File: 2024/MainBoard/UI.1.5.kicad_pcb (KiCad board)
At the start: 2 copper layers, 105.9 x 122.4 mm, 31 parts, among them J1 debug, Y2 Crystal_GND24

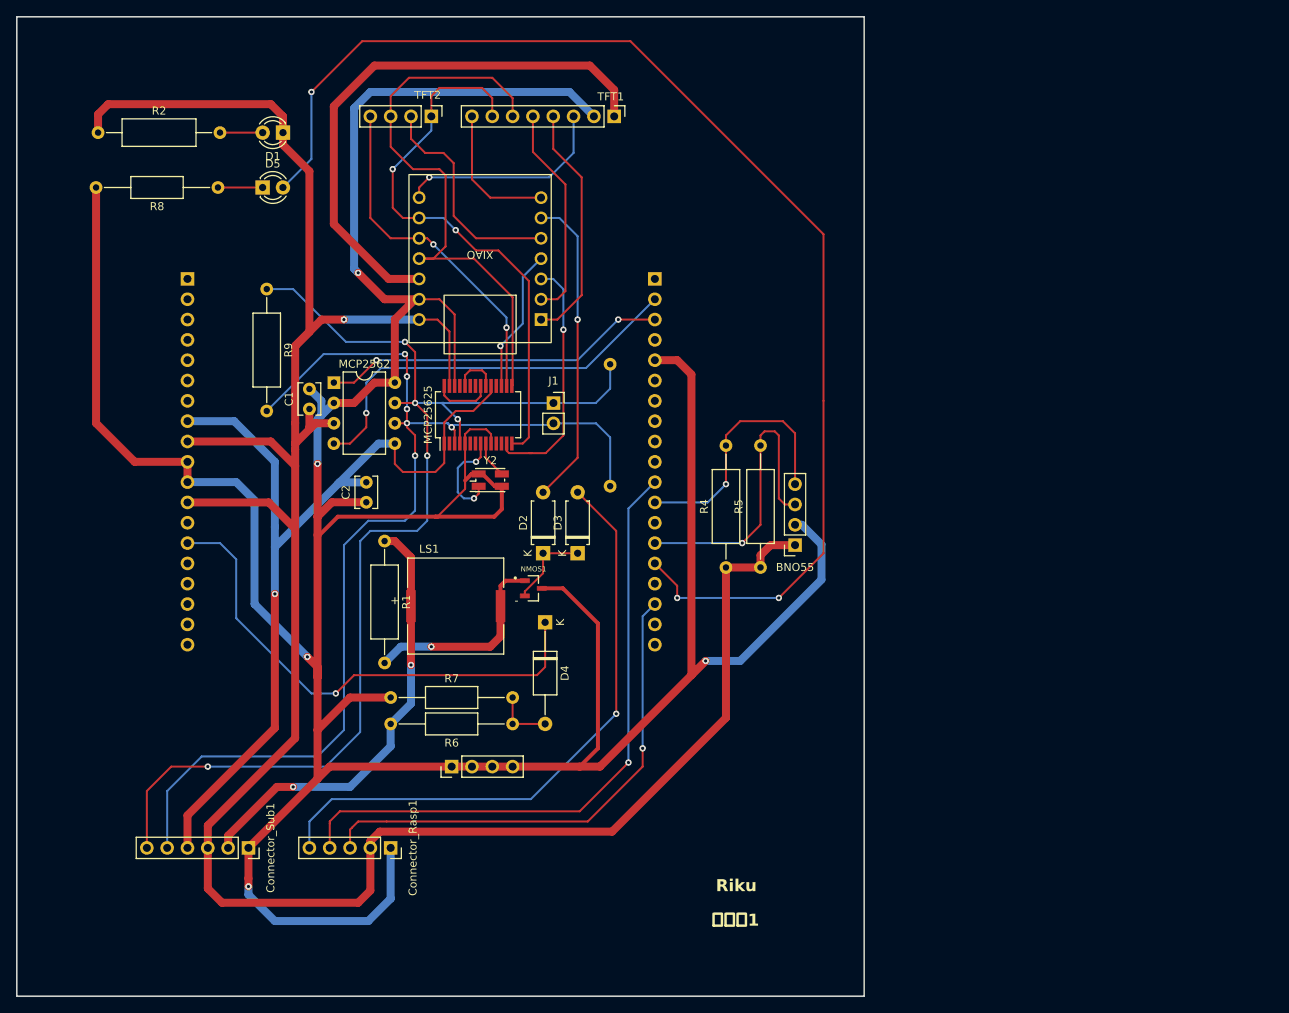
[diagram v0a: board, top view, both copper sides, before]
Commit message: アートワークした
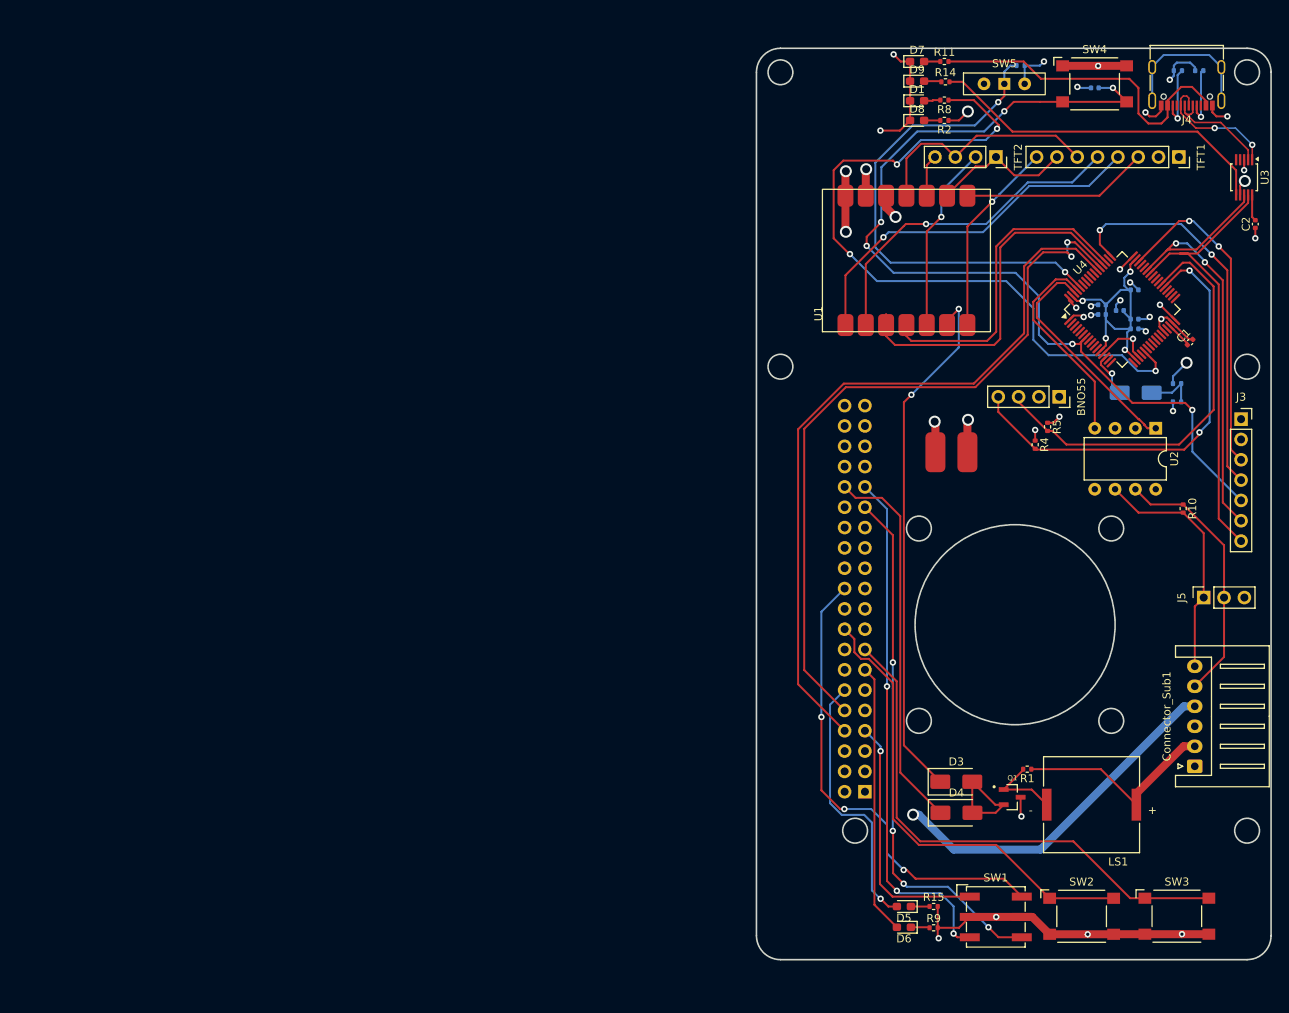
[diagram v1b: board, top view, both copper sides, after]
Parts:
- removed Connector_Rasp1: ~, Connector_PinSocket_2.54mm:PinSocket_1x05_P2.54mm_Vertical
- removed F446RE_CN10, F446RE_CN7: ~, Connector_PinSocket_2.54mm:PinSocket_1x19_P2.54mm_Vertical
- removed MCP2562: MCP2562-E-P, Package_DIP:DIP-8_W7.62mm
- removed MCP25625: MCP25625-x-SS, Package_SO:SSOP-28_5.3x10.2mm_P0.65mm
- removed NMOS1: BSS138, NMOS:SOT95P240X111-3N
- removed TFT3: ~, Connector_PinHeader_2.54mm:PinHeader_1x04_P2.54mm_Vertical
- removed XIAO: MOUDLE-SEEEDUINO-XIAO, XIAO:MOUDLE14P-2.54-21X17.8MM
- removed Y2: Crystal_GND24, Oscillator:Oscillator_SMD_EuroQuartz_XO32-4Pin_3.2x2.5mm_HandSoldering
- added C3: 4.7uF, Capacitor_SMD:C_0402_1005Metric, B.Cu at (225.8, 67.5)
- added C4: 0.1uF, Capacitor_SMD:C_0402_1005Metric, B.Cu at (223.5, 68.0)
- added C5: 0.1uF, Capacitor_SMD:C_0402_1005Metric, B.Cu at (223.5, 66.7)
- added C6: 0.1uF, Capacitor_SMD:C_0402_1005Metric, B.Cu at (227.6, 68.5)
- added C7: 0.1uF, Capacitor_SMD:C_0402_1005Metric, B.Cu at (227.6, 64.9)
- added C8: 0.1uF, Capacitor_SMD:C_0402_1005Metric, B.Cu at (227.6, 69.7)
- added C9: 0.1uF, Capacitor_SMD:C_0402_1005Metric, B.Cu at (222.6, 39.6)
- added D6: LED_Ras2, LED_SMD:LED_0603_1608Metric_Pad1.05x0.95mm_HandSolder, F.Cu at (198.8, 144.5)
- added D7: LED_USB, LED_SMD:LED_0603_1608Metric_Pad1.05x0.95mm_HandSolder, F.Cu at (200.4, 36.3)
- added D8: LED_volt, LED_SMD:LED_0603_1608Metric_Pad1.05x0.95mm_HandSolder, F.Cu at (200.4, 43.7)
- added D9: LED_Debug, LED_SMD:LED_0603_1608Metric_Pad1.05x0.95mm_HandSolder, F.Cu at (200.4, 38.8)
- added J2: fan, pad:fan_pad, F.Cu at (204.7, 85.2)
- added J3: Debug, Connector_PinSocket_2.54mm:PinSocket_1x07_P2.54mm_Vertical, F.Cu at (240.9, 81.0)
- added J4: USB_C_Receptacle_USB2.0_16P, Connector_USB:USB_C_Receptacle_G-Switch_GT-USB-7010ASV, F.Cu at (234.1, 38.1)
- added J5: Can_debug, Connector_PinSocket_2.54mm:PinSocket_1x03_P2.54mm_Vertical, F.Cu at (236.2, 103.3)
- added Q1: NMOS, NMOS:SOT95P240X111-3N, F.Cu at (212.3, 128.3)
- added R10: 120, Resistor_SMD:R_0402_1005Metric, F.Cu at (233.7, 92.2)
- added R11: 120, Resistor_SMD:R_0402_1005Metric, F.Cu at (203.8, 36.3)
- added R12: 5.1k, Resistor_SMD:R_0402_1005Metric, B.Cu at (235.7, 37.5)
- added R13: 5.1k, Resistor_SMD:R_0402_1005Metric, B.Cu at (233.0, 37.5)
- added R14: 120, Resistor_SMD:R_0402_1005Metric, F.Cu at (204.0, 38.9)
- added R15: R, Resistor_SMD:R_0402_1005Metric, F.Cu at (202.5, 141.9)
- added SW1: SW_Coded_SH-7050, Button_Switch_SMD:Nidec_Copal_SH-7010A, F.Cu at (210.3, 143.2)
- added SW2: Ras_1, Button_Switch_SMD:SW_SPST_Omron_B3FS-100xP, F.Cu at (221.0, 143.2)
- added SW3: Ras_2, Button_Switch_SMD:SW_SPST_Omron_B3FS-100xP, F.Cu at (232.9, 143.2)
- added SW4: NRST, Button_Switch_SMD:SW_SPST_Omron_B3FS-100xP, F.Cu at (222.6, 39.1)
- added SW5: Boot, Button_Switch_THT:SW_Slide-03_Wuerth-WS-SLTV_10x2.5x6.4_P2.54mm, F.Cu at (211.3, 39.1)
- added U1: MOUDLE-SEEEDUINO-XIAO, XIAO:MOUDLE14P-SMD-2.54-21X17.8MM, F.Cu at (209.6, 70.1)
- added U2: MCP2562-E-P, Package_DIP:DIP-8_W7.62mm, F.Cu at (230.3, 82.2)
- added U3: CH340E, Package_SO:MSOP-10_3x3mm_P0.5mm, F.Cu at (241.3, 50.8)
- added U4: STM32F446RETx, Package_QFP:LQFP-64_10x10mm_P0.5mm, F.Cu at (226.1, 67.3)
- C1: value C -> 4.7u; footprint Capacitor_THT:C_Disc_D3.8mm_W2.6mm_P2.50mm -> Capacitor_SMD:C_0402_1005Metric
- C2: value C -> 0.1uF; footprint Capacitor_THT:C_Disc_D3.8mm_W2.6mm_P2.50mm -> Capacitor_SMD:C_0402_1005Metric
- Connector_Sub1: footprint Connector_PinSocket_2.54mm:PinSocket_1x06_P2.54mm_Vertical -> Connector_JST:JST_XH_S6B-XH-A_1x06_P2.50mm_Horizontal
- D1: value LED -> LED_main; footprint LED_THT:LED_D3.0mm -> LED_SMD:LED_0603_1608Metric_Pad1.05x0.95mm_HandSolder
- D2: value D -> SS210; footprint Diode_THT:D_A-405_P7.62mm_Horizontal -> Diode_SMD:D_SMA; moved to B.Cu
- D3: value D -> SS210; footprint Diode_THT:D_A-405_P7.62mm_Horizontal -> Diode_SMD:D_SMA
- D4: value D -> SS210; footprint Diode_THT:D_A-405_P12.70mm_Horizontal -> Diode_SMD:D_SMA
- D5: value LED -> LED_Ras1; footprint LED_THT:LED_D3.0mm -> LED_SMD:LED_0603_1608Metric_Pad1.05x0.95mm_HandSolder
- J1: value debug -> Raspberry_Pi_2_3; footprint Connector_PinSocket_2.54mm:PinSocket_1x02_P2.54mm_Vertical -> Connector_PinSocket_2.54mm:PinSocket_2x20_P2.54mm_Vertical; moved to B.Cu
- R1, R3, R4, R5: footprint Resistor_THT:R_Axial_DIN0309_L9.0mm_D3.2mm_P15.24mm_Horizontal -> Resistor_SMD:R_0402_1005Metric
- R2: value 600R -> 300; footprint Resistor_THT:R_Axial_DIN0309_L9.0mm_D3.2mm_P15.24mm_Horizontal -> Resistor_SMD:R_0402_1005Metric
- R6, R7: footprint Resistor_THT:R_Axial_DIN0207_L6.3mm_D2.5mm_P15.24mm_Horizontal -> Resistor_SMD:R_0402_1005Metric; moved to B.Cu
- R8: footprint Resistor_THT:R_Axial_DIN0207_L6.3mm_D2.5mm_P15.24mm_Horizontal -> Resistor_SMD:R_0402_1005Metric
- R9: value 120 -> R; footprint Resistor_THT:R_Axial_DIN0309_L9.0mm_D3.2mm_P15.24mm_Horizontal -> Resistor_SMD:R_0402_1005Metric
- TFT1: footprint Connector_PinHeader_2.54mm:PinHeader_1x08_P2.54mm_Vertical -> Connector_PinSocket_2.54mm:PinSocket_1x08_P2.54mm_Vertical
- TFT2: footprint Connector_PinHeader_2.54mm:PinHeader_1x04_P2.54mm_Vertical -> Connector_PinSocket_2.54mm:PinSocket_1x04_P2.54mm_Vertical
- moved D5 120.4 mm to (198.8, 141.9), turned to 180 degrees
- moved Connector_Sub1 118.7 mm to (235.1, 124.4), turned to 90 degrees
- moved C2 116.4 mm to (242.7, 56.6)
- moved R9 115.4 mm to (202.5, 144.6), turned to 0 degrees
- moved C1 110.4 mm to (234.5, 71.4), turned to 45 degrees
- moved R2 105.8 mm to (203.8, 43.7), turned to 180 degrees
- moved R7 105.0 mm to (232.9, 78.9)
- moved R6 93.3 mm to (232.9, 76.6)
- moved R8 91.5 mm to (203.8, 41.1)
- moved R1 85.2 mm to (214.2, 124.8), turned to 180 degrees
- moved LS1 83.3 mm to (222.2, 129.2), turned to 180 degrees
- moved D1 79.4 mm to (200.4, 41.2), turned to 0 degrees
- moved D2 76.7 mm to (227.7, 77.7), turned to 180 degrees
- moved TFT2 70.8 mm to (210.3, 48.3)
- moved TFT1 70.8 mm to (233.1, 48.3)
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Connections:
- C1 pad 1: +5V -> Net-(U4-VCAP_1)
- C2 pad 2: +3.3V -> Net-(U3-V3)
- D1 pad 1: +5V -> GND
- D2 pad 2: UI_Audio -> Volt_SIG
- D3 pad 1: Net-(D2-K) -> UI_Audio
- D3 pad 2: Ras_Audio -> Net-(D3-A)
- D4 pad 1: Volt_SIG -> Ras_Audio
- D4 pad 2: Net-(D4-A) -> Net-(D3-A)
- D5 pad 2: Main_LED -> LED1
- J1 pad 1: CANH -> +3.3V
- J1 pad 2: CANL -> +5V
- R2 pad 2: Net-(D1-A) -> Net-(D8-A)
- R3 pad 1: CANH -> Net-(SW5-B)
- R3 pad 2: CANL -> GND
- R6 pad 1: Net-(D4-A) -> Net-(D2-K)
- R7 pad 2: Net-(D4-A) -> Net-(D2-K)
- R8 pad 1: Net-(D5-K) -> Main_LED
- R8 pad 2: GND -> Net-(D1-A)
- R9 pad 1: CANH -> Net-(D6-K)
- R9 pad 2: CANL -> GND
- TFT1 pad 1: 3.3V -> +3.3V
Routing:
- net GND: track 494.5 -> 135.7 mm, vias 5 -> 23
- net +3.3V: track 112.8 -> 302.4 mm, vias 1 -> 13
- net CANH: track 150.6 -> 30.5 mm, vias 5 -> 0
- net NRST: track 0.00 -> 117.3 mm, vias 0 -> 6
- net CANL: track 143.3 -> 33.4 mm, vias 6 -> 0
- net 3.3V: track 70.0 -> 0.00 mm
- net R2: track 0.00 -> 66.6 mm, vias 0 -> 4
- net SW2: track 0.00 -> 65.9 mm
- net R3: track 0.00 -> 65.7 mm, vias 0 -> 3
- net Main_LED: track 156.0 -> 92.1 mm, vias 3 -> 4
- net Net-(SW5-B): track 0.00 -> 62.7 mm, vias 0 -> 2
- net R4: track 0.00 -> 59.1 mm, vias 0 -> 3
- net SW1: track 0.00 -> 58.5 mm
- net Volt_SIG: track 63.8 -> 5.86 mm
- net ST_TX: track 0.00 -> 57.3 mm, vias 0 -> 2
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- added copper zone on In1.Cu, net +3.3V
- added copper zone on In2.Cu, net GND
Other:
- board size 105.9 x 122.4 mm -> 64.3 x 113.9 mm
- copper layers 2 -> 4
- board text removed: "Riku"
- board text removed: "検証用1"
